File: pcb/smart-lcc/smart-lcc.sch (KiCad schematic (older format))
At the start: 12 parts, among them J1 Control board connector, J2 Aux connector, J3 Conn_01x24 (mirrored), SW1 SW_Push, SW2 SW_Push, U1 ABX00027

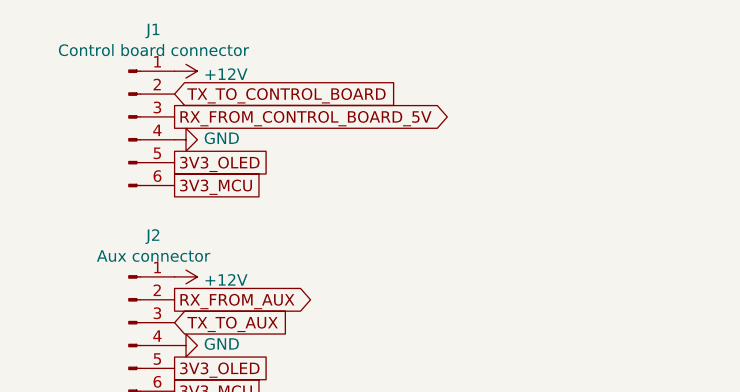
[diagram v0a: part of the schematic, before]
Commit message: WIP
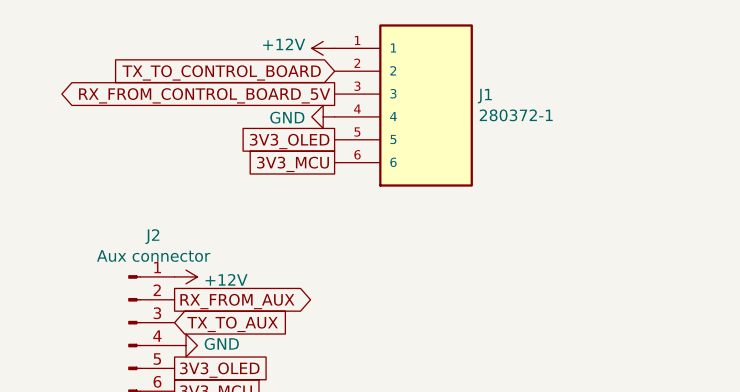
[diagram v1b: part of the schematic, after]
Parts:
- removed J1: Control board connector, Connector_PinHeader_2.54mm:PinHeader_1x06_P2.54mm_Vertical, symbol Connector:Conn_01x06_Male
- added J1: 280372-1, TE_280372-1, symbol TE_280372-1:280372-1
- C3: footprint Capacitor_SMD:C_0603_1608Metric -> Capacitor_SMD:C_1206_3216Metric
- R1, R2: footprint Resistor_SMD:R_0402_1005Metric -> Resistor_SMD:R_0603_1608Metric
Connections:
- net +12V: now also J1.1
- net 3V3_MCU: now also J1.6
- net 3V3_OLED: now also J1.5
- net GND: now also J1.4
- net RX_FROM_CONTROL_BOARD_5V: now also J1.3
- net TX_TO_CONTROL_BOARD: now also J1.2
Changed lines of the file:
@@
 F 0 "R2" V 1243 3700 50  0000 C CNN
 F 1 "3K3" V 1334 3700 50  0000 C CNN
-F 2 "Resistor_SMD:R_0402_1005Metric" V 1380 3700 50  0001 C CNN
+F 2 "Resistor_SMD:R_0603_1608Metric" V 1380 3700 50  0001 C CNN
 F 3 "~" H 1450 3700 50  0001 C CNN
 	1    1450 3700
@@
 F 0 "R1" V 943 3700 50  0000 C CNN
 F 1 "2K2" V 1034 3700 50  0000 C CNN
-F 2 "Resistor_SMD:R_0402_1005Metric" V 1080 3700 50  0001 C CNN
+F 2 "Resistor_SMD:R_0603_1608Metric" V 1080 3700 50  0001 C CNN
 F 3 "~" H 1150 3700 50  0001 C CNN
 	1    1150 3700
 	0    1    1    0
 $EndComp
-Text GLabel 1050 1050 2    50   Output ~ 0
+Text GLabel 1750 950  0    50   Output ~ 0
 RX_FROM_CONTROL_BOARD_5V
-Text GLabel 1050 950  2    50   Input ~ 0
+Text GLabel 1750 850  0    50   Input ~ 0
 TX_TO_CONTROL_BOARD
 $Comp
@@
 Text GLabel 1050 2150 2    50   UnSpc ~ 0
 3V3_OLED
-Text GLabel 1050 1250 2    50   UnSpc ~ 0
+Text GLabel 1750 1150 0    50   UnSpc ~ 0
 3V3_OLED
 $Comp
@@
 L power:+12V #PWR0103
 U 1 1 60D7DDC1
-P 1050 850
-F 0 "#PWR0103" H 1050 700 50  0001 C CNN
-F 1 "+12V" V 1065 978 50  0000 L CNN
-F 2 "" H 1050 850 50  0001 C CNN
-F 3 "" H 1050 850 50  0001 C CNN
-	1    1050 850
-	0    1    1    0
+P 1750 750
+F 0 "#PWR0103" H 1750 600 50  0001 C CNN
+F 1 "+12V" V 1765 878 50  0000 L CNN
+F 2 "" H 1750 750 50  0001 C CNN
+F 3 "" H 1750 750 50  0001 C CNN
+	1    1750 750
+	0    -1   -1   0
 $EndComp
 $Comp
@@
 L power:GND #PWR0101
 U 1 1 60D7C577
-P 1050 1150
-F 0 "#PWR0101" H 1050 900 50  0001 C CNN
-F 1 "GND" V 1055 1022 50  0000 R CNN
-F 2 "" H 1050 1150 50  0001 C CNN
-F 3 "" H 1050 1150 50  0001 C CNN
-	1    1050 1150
-	0    -1   -1   0
+P 1750 1050
+F 0 "#PWR0101" H 1750 800 50  0001 C CNN
+F 1 "GND" V 1755 922 50  0000 R CNN
+F 2 "" H 1750 1050 50  0001 C CNN
+F 3 "" H 1750 1050 50  0001 C CNN
+	1    1750 1050
+	0    1    1    0
 $EndComp
 $Comp
@@
 Text GLabel 4350 1950 0    50   UnSpc ~ 0
 3V3_OLED
-$Comp
-L Connector:Conn_01x06_Male J1
-U 1 1 60D7884D
-P 850 1050
-F 0 "J1" H 958 1431 50  0000 C CNN
-F 1 "Control board connector" H 958 1340 50  0000 C CNN
-F 2 "Connector_PinHeader_2.54mm:PinHeader_1x06_P2.54mm_Vertical" H 850 1050 50  0001 C CNN
-F 3 "~" H 850 1050 50  0001 C CNN
-	1    850  1050
-	1    0    0    -1
-$EndComp
-Text GLabel 1050 1350 2    50   UnSpc ~ 0
+Text GLabel 1750 1250 0    50   UnSpc ~ 0
 3V3_MCU
 Text GLabel 1050 2250 2    50   UnSpc ~ 0
@@
 F 0 "C3" V 3621 4300 50  0000 C CNN
 F 1 "0.1 µF / 25V, X7R" V 3712 4300 50  0000 C CNN
-F 2 "Capacitor_SMD:C_0603_1608Metric" H 3850 4300 50  0001 C CNN
+F 2 "Capacitor_SMD:C_1206_3216Metric" H 3850 4300 50  0001 C CNN
 F 3 "~" H 3850 4300 50  0001 C CNN
 	1    3850 4300
@@
 	0    1    1    0
 $EndComp
+$Comp
+L TE_280372-1:280372-1 J1
+U 1 1 60D8FA50
+P 2150 1050
+F 0 "J1" H 2380 1146 50  0000 L CNN
+F 1 "280372-1" H 2380 1055 50  0000 L CNN
+F 2 "TE_280372-1" H 2150 1050 50  0001 L BNN
+F 3 "" H 2150 1050 50  0001 L BNN
+F 4 "Connector" H 2150 1050 50  0001 L BNN "Product_Type"
+F 5 "2.54 mm[.1 in]" H 2150 1050 50  0001 L BNN "Centerline_Pitch"
+F 6 "6" H 2150 1050 50  0001 L BNN "Number_of_Positions"
+F 7 "280372-1" H 2150 1050 50  0001 L BNN "Comment"
+F 8 "Compliant" H 2150 1050 50  0001 L BNN "EU_RoHS_Compliance"
+	1    2150 1050
+	1    0    0    -1
+$EndComp
 $EndSCHEMATC

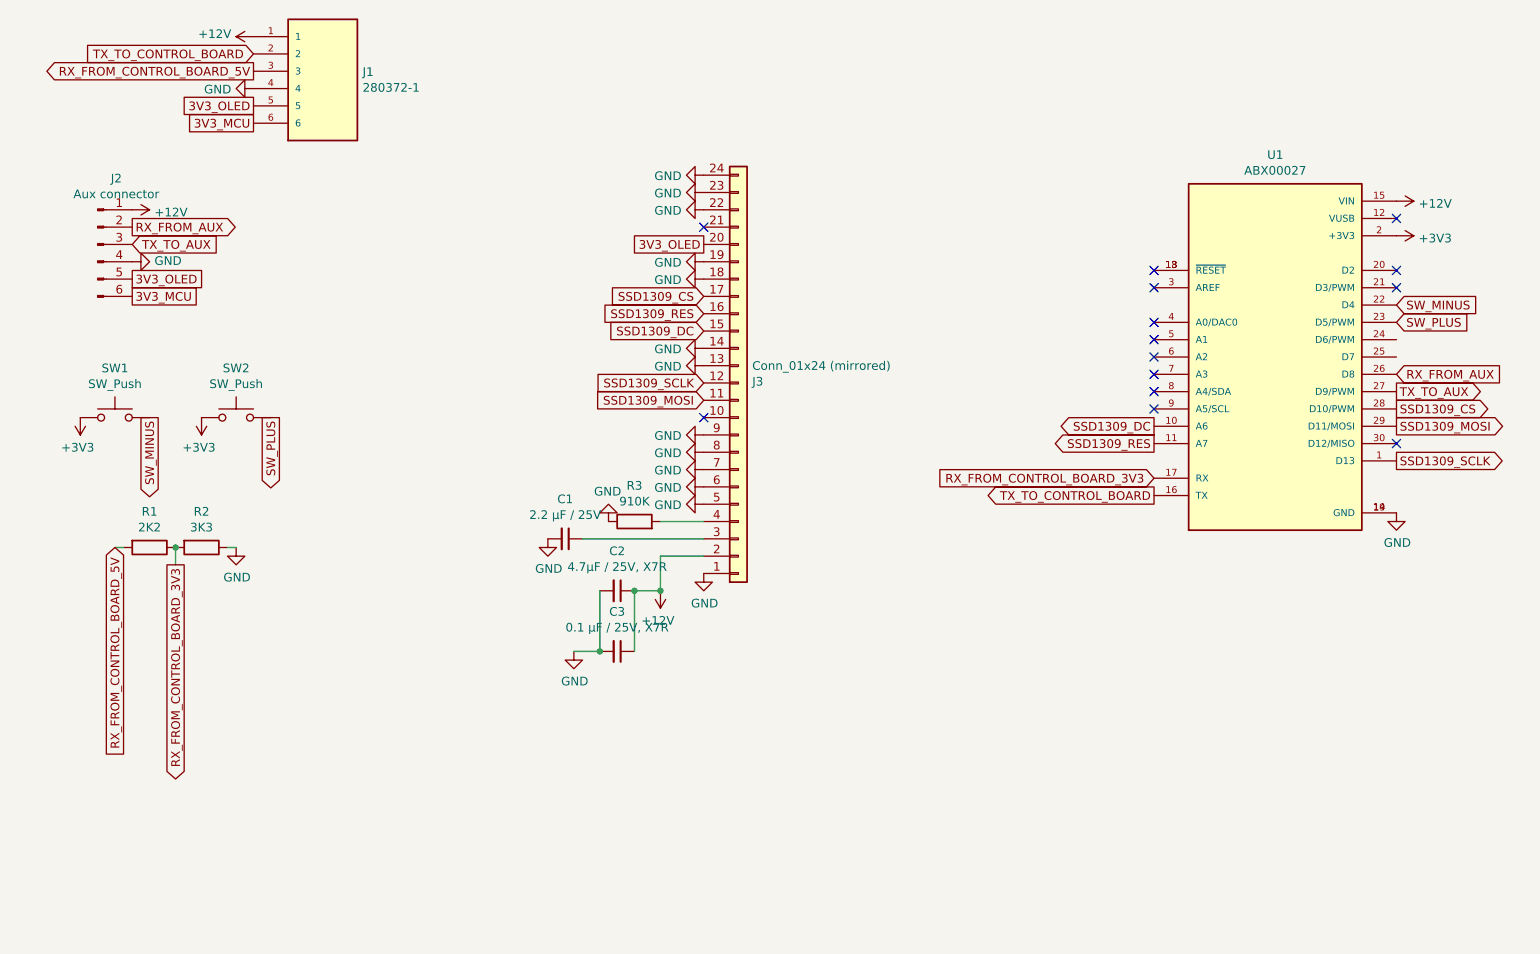
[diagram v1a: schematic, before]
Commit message: WIP
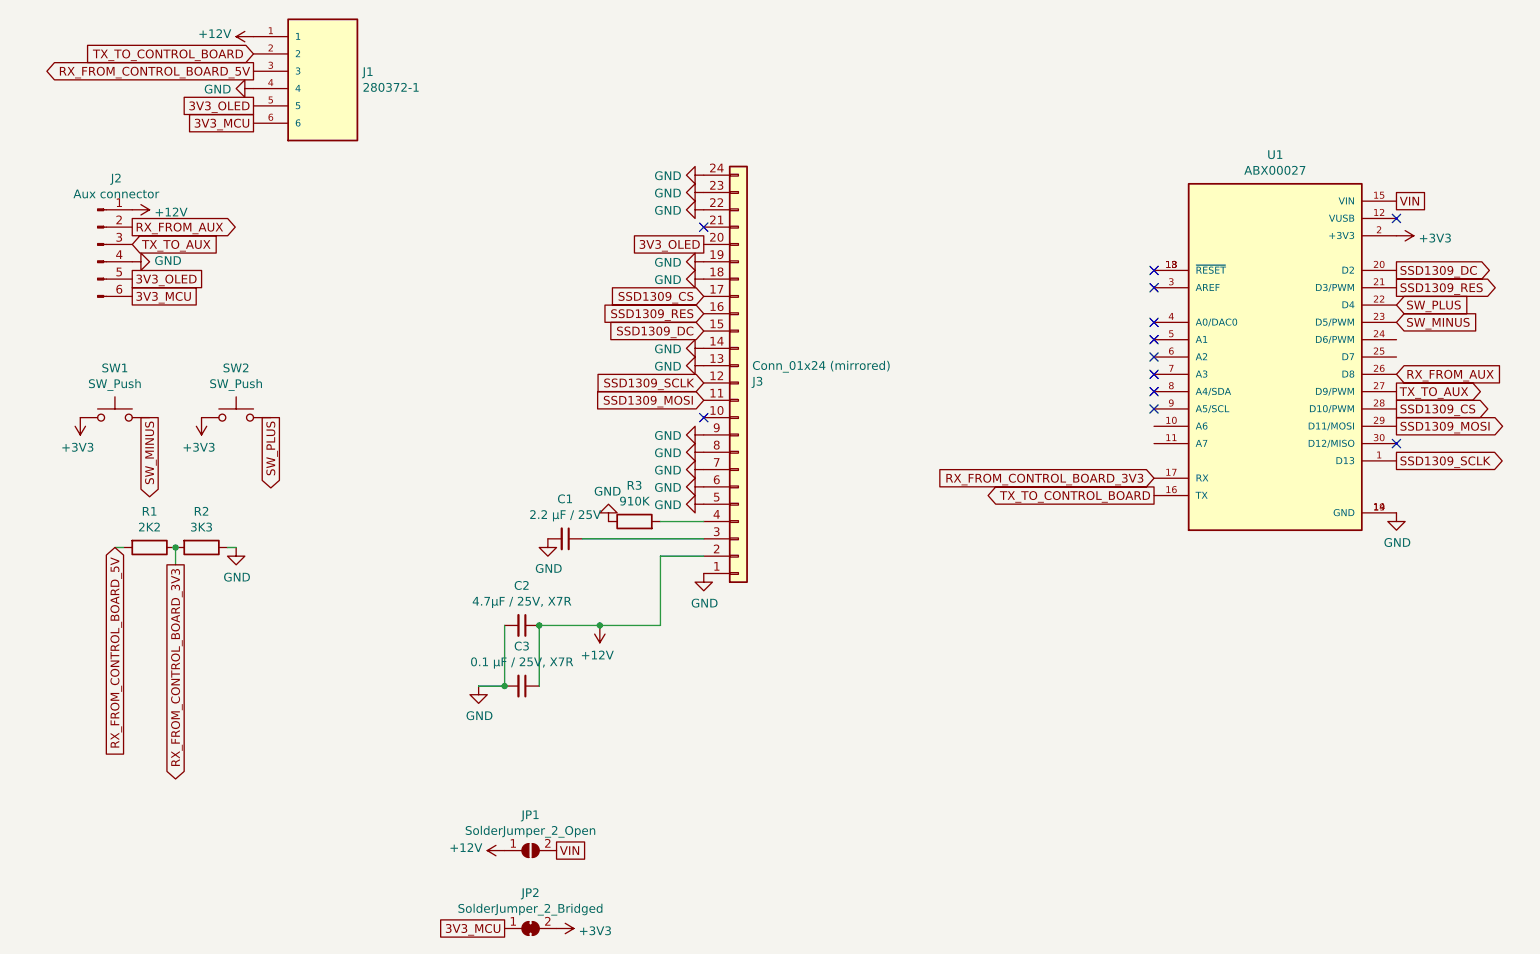
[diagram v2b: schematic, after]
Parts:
- added JP1: SolderJumper_2_Open, Jumper:SolderJumper-2_P1.3mm_Open_RoundedPad1.0x1.5mm, symbol Jumper:SolderJumper_2_Open
- added JP2: SolderJumper_2_Bridged, Jumper:SolderJumper-2_P1.3mm_Bridged_RoundedPad1.0x1.5mm, symbol Jumper:SolderJumper_2_Bridged
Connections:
- net +12V: now also JP1.1 (A); no longer U1.15 (VIN)
- net +3V3: now also JP2.2 (B)
- net 3V3_MCU: now also JP2.1 (A)
- net SSD1309_DC: now also U1.20 (D2); no longer U1.10 (A6)
- net SSD1309_RES: now also U1.21 (D3/PWM); no longer U1.11 (A7)
- net SW_MINUS: now also U1.23 (D5/PWM); no longer U1.22 (D4)
- net SW_PLUS: now also U1.22 (D4); no longer U1.23 (D5/PWM)
- new net VIN: JP1.2 (B), U1.15 (VIN)
- no-connect marks 14 -> 12
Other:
- moved on the sheet: C2, C3
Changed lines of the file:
@@
 Text GLabel 8350 3000 2    50   Output ~ 0
 SSD1309_MOSI
-Text GLabel 6950 3000 0    50   Output ~ 0
+Text GLabel 8350 2100 2    50   Output ~ 0
 SSD1309_DC
-Text GLabel 6950 3100 0    50   Output ~ 0
+Text GLabel 8350 2200 2    50   Output ~ 0
 SSD1309_RES
 Text GLabel 8350 2900 2    50   Output ~ 0
@@
 L power:+12V #PWR0130
 U 1 1 60D9A09F
-P 8350 1700
-F 0 "#PWR0130" H 8350 1550 50  0001 C CNN
-F 1 "+12V" V 8365 1828 50  0000 L CNN
-F 2 "" H 8350 1700 50  0001 C CNN
-F 3 "" H 8350 1700 50  0001 C CNN
-	1    8350 1700
-	0    1    1    0
+P 3200 5450
+F 0 "#PWR0130" H 3200 5300 50  0001 C CNN
+F 1 "+12V" V 3215 5578 50  0000 L CNN
+F 2 "" H 3200 5450 50  0001 C CNN
+F 3 "" H 3200 5450 50  0001 C CNN
+	1    3200 5450
+	0    -1   -1   0
 $EndComp
 NoConn ~ 8350 1800
@@
 Text GLabel 1850 2950 3    50   Output ~ 0
 SW_PLUS
+Text GLabel 8350 2400 2    50   Input ~ 0
+SW_MINUS
 Text GLabel 8350 2300 2    50   Input ~ 0
-SW_MINUS
-Text GLabel 8350 2400 2    50   Input ~ 0
 SW_PLUS
-NoConn ~ 8350 2200
-NoConn ~ 8350 2100
 NoConn ~ 6950 2100
 NoConn ~ 6950 2200
@@
 NoConn ~ 4350 2950
 Wire Wire Line
-	3750 3950 3750 4300
-Connection ~ 3950 3950
+	3200 4150 3200 4500
+Connection ~ 3400 4150
 Wire Wire Line
-	3950 3950 3950 4300
-Connection ~ 4100 3950
-Wire Wire Line
-	4100 3950 4100 3750
-Wire Wire Line
-	4100 3950 3950 3950
+	3400 4150 3400 4500
 $Comp
 L power:+12V #PWR0125
 U 1 1 60D94DE0
-P 4100 3950
-F 0 "#PWR0125" H 4100 3800 50  0001 C CNN
-F 1 "+12V" H 4115 4123 50  0000 C CNN
-F 2 "" H 4100 3950 50  0001 C CNN
-F 3 "" H 4100 3950 50  0001 C CNN
-	1    4100 3950
+P 3750 4150
+F 0 "#PWR0125" H 3750 4000 50  0001 C CNN
+F 1 "+12V" H 3765 4323 50  0000 C CNN
+F 2 "" H 3750 4150 50  0001 C CNN
+F 3 "" H 3750 4150 50  0001 C CNN
+	1    3750 4150
 	-1   0    0    1
 $EndComp
-Connection ~ 3750 4300
+Connection ~ 3200 4500
 Wire Wire Line
-	3600 4300 3750 4300
+	3050 4500 3200 4500
 $Comp
 L power:GND #PWR0124
 U 1 1 60D925DE
-P 3600 4300
-F 0 "#PWR0124" H 3600 4050 50  0001 C CNN
-F 1 "GND" H 3605 4127 50  0000 C CNN
-F 2 "" H 3600 4300 50  0001 C CNN
-F 3 "" H 3600 4300 50  0001 C CNN
-	1    3600 4300
+P 3050 4500
+F 0 "#PWR0124" H 3050 4250 50  0001 C CNN
+F 1 "GND" H 3055 4327 50  0000 C CNN
+F 2 "" H 3050 4500 50  0001 C CNN
+F 3 "" H 3050 4500 50  0001 C CNN
+	1    3050 4500
 	1    0    0    -1
 $EndComp
@@
 L Device:C_Small C3
 U 1 1 60D9151C
-P 3850 4300
-F 0 "C3" V 3621 4300 50  0000 C CNN
-F 1 "0.1 µF / 25V, X7R" V 3712 4300 50  0000 C CNN
-F 2 "Capacitor_SMD:C_1206_3216Metric" H 3850 4300 50  0001 C CNN
-F 3 "~" H 3850 4300 50  0001 C CNN
-	1    3850 4300
+P 3300 4500
+F 0 "C3" V 3071 4500 50  0000 C CNN
+F 1 "0.1 µF / 25V, X7R" V 3162 4500 50  0000 C CNN
+F 2 "Capacitor_SMD:C_1206_3216Metric" H 3300 4500 50  0001 C CNN
+F 3 "~" H 3300 4500 50  0001 C CNN
+	1    3300 4500
 	0    1    1    0
 $EndComp
@@
 L Device:C_Small C2
 U 1 1 60D8F384
-P 3850 3950
-F 0 "C2" V 3621 3950 50  0000 C CNN
-F 1 "4.7µF / 25V, X7R" V 3712 3950 50  0000 C CNN
-F 2 "Capacitor_SMD:C_1206_3216Metric" H 3850 3950 50  0001 C CNN
-F 3 "~" H 3850 3950 50  0001 C CNN
-	1    3850 3950
+P 3300 4150
+F 0 "C2" V 3071 4150 50  0000 C CNN
+F 1 "4.7µF / 25V, X7R" V 3162 4150 50  0000 C CNN
+F 2 "Capacitor_SMD:C_1206_3216Metric" H 3300 4150 50  0001 C CNN
+F 3 "~" H 3300 4150 50  0001 C CNN
+	1    3300 4150
 	0    1    1    0
 $EndComp
@@
 	1    0    0    -1
 $EndComp
+Text GLabel 8350 1700 2    50   UnSpc ~ 0
+VIN
+$Comp
+L Jumper:SolderJumper_2_Open JP1
+U 1 1 60DA70BB
+P 3350 5450
+F 0 "JP1" H 3350 5655 50  0000 C CNN
+F 1 "SolderJumper_2_Open" H 3350 5564 50  0000 C CNN
+F 2 "Jumper:SolderJumper-2_P1.3mm_Open_RoundedPad1.0x1.5mm" H 3350 5450 50  0001 C CNN
+F 3 "~" H 3350 5450 50  0001 C CNN
+	1    3350 5450
+	1    0    0    -1
+$EndComp
+Text GLabel 3500 5450 2    50   UnSpc ~ 0
+VIN
+$Comp
+L Jumper:SolderJumper_2_Bridged JP2
+U 1 1 60DA997A
+P 3350 5900
+F 0 "JP2" H 3350 6105 50  0000 C CNN
+F 1 "SolderJumper_2_Bridged" H 3350 6014 50  0000 C CNN
+F 2 "Jumper:SolderJumper-2_P1.3mm_Bridged_RoundedPad1.0x1.5mm" H 3350 5900 50  0001 C CNN
+F 3 "~" H 3350 5900 50  0001 C CNN
+	1    3350 5900
+	1    0    0    -1
+$EndComp
+Text GLabel 3200 5900 0    50   UnSpc ~ 0
+3V3_MCU
+$Comp
+L power:+3V3 #PWR0111
+U 1 1 60DAA2F1
+P 3500 5900
+F 0 "#PWR0111" H 3500 5750 50  0001 C CNN
+F 1 "+3V3" V 3515 6028 50  0000 L CNN
+F 2 "" H 3500 5900 50  0001 C CNN
+F 3 "" H 3500 5900 50  0001 C CNN
+	1    3500 5900
+	0    1    1    0
+$EndComp
+Wire Wire Line
+	4100 3750 4100 4150
+Connection ~ 3750 4150
+Wire Wire Line
+	3400 4150 3750 4150
+Wire Wire Line
+	3750 4150 4100 4150
 $EndSCHEMATC

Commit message: Getting ready to manufacture PCB
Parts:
- R1, R2, R3: footprint Resistor_SMD:R_0603_1608Metric -> Resistor_SMD:R_1206_3216Metric
- SW1, SW2: footprint Button_Switch_SMD:SW_Push_1P1T_NO_6x6mm_H9.5mm -> SW_Push_ADTSMW65:ADTSMW65
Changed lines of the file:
@@
 F 0 "R2" V 1243 3700 50  0000 C CNN
 F 1 "3K3" V 1334 3700 50  0000 C CNN
-F 2 "Resistor_SMD:R_0603_1608Metric" V 1380 3700 50  0001 C CNN
+F 2 "Resistor_SMD:R_1206_3216Metric" V 1380 3700 50  0001 C CNN
 F 3 "~" H 1450 3700 50  0001 C CNN
 	1    1450 3700
@@
 F 0 "R1" V 943 3700 50  0000 C CNN
 F 1 "2K2" V 1034 3700 50  0000 C CNN
-F 2 "Resistor_SMD:R_0603_1608Metric" V 1080 3700 50  0001 C CNN
+F 2 "Resistor_SMD:R_1206_3216Metric" V 1080 3700 50  0001 C CNN
 F 3 "~" H 1150 3700 50  0001 C CNN
 	1    1150 3700
@@
 F 0 "SW2" H 1650 3235 50  0000 C CNN
 F 1 "SW_Push" H 1650 3144 50  0000 C CNN
-F 2 "Button_Switch_SMD:SW_Push_1P1T_NO_6x6mm_H9.5mm" H 1650 3150 50  0001 C CNN
+F 2 "SW_Push_ADTSMW65:ADTSMW65" H 1650 3150 50  0001 C CNN
 F 3 "~" H 1650 3150 50  0001 C CNN
 	1    1650 2950
@@
 F 0 "SW1" H 950 3235 50  0000 C CNN
 F 1 "SW_Push" H 950 3144 50  0000 C CNN
-F 2 "Button_Switch_SMD:SW_Push_1P1T_NO_6x6mm_H9.5mm" H 950 3150 50  0001 C CNN
+F 2 "SW_Push_ADTSMW65:ADTSMW65" H 950 3150 50  0001 C CNN
 F 3 "~" H 950 3150 50  0001 C CNN
 	1    950  2950
@@
 F 0 "R3" V 4157 3550 50  0000 C CNN
 F 1 "910K" V 4066 3550 50  0000 C CNN
-F 2 "Resistor_SMD:R_0603_1608Metric" V 3880 3550 50  0001 C CNN
+F 2 "Resistor_SMD:R_1206_3216Metric" V 3880 3550 50  0001 C CNN
 F 3 "~" H 3950 3550 50  0001 C CNN
 	1    3950 3550
